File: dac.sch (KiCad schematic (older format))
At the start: 46 parts, among them U15 OPA4172, U4 OPA4172, U8 DAC8568C

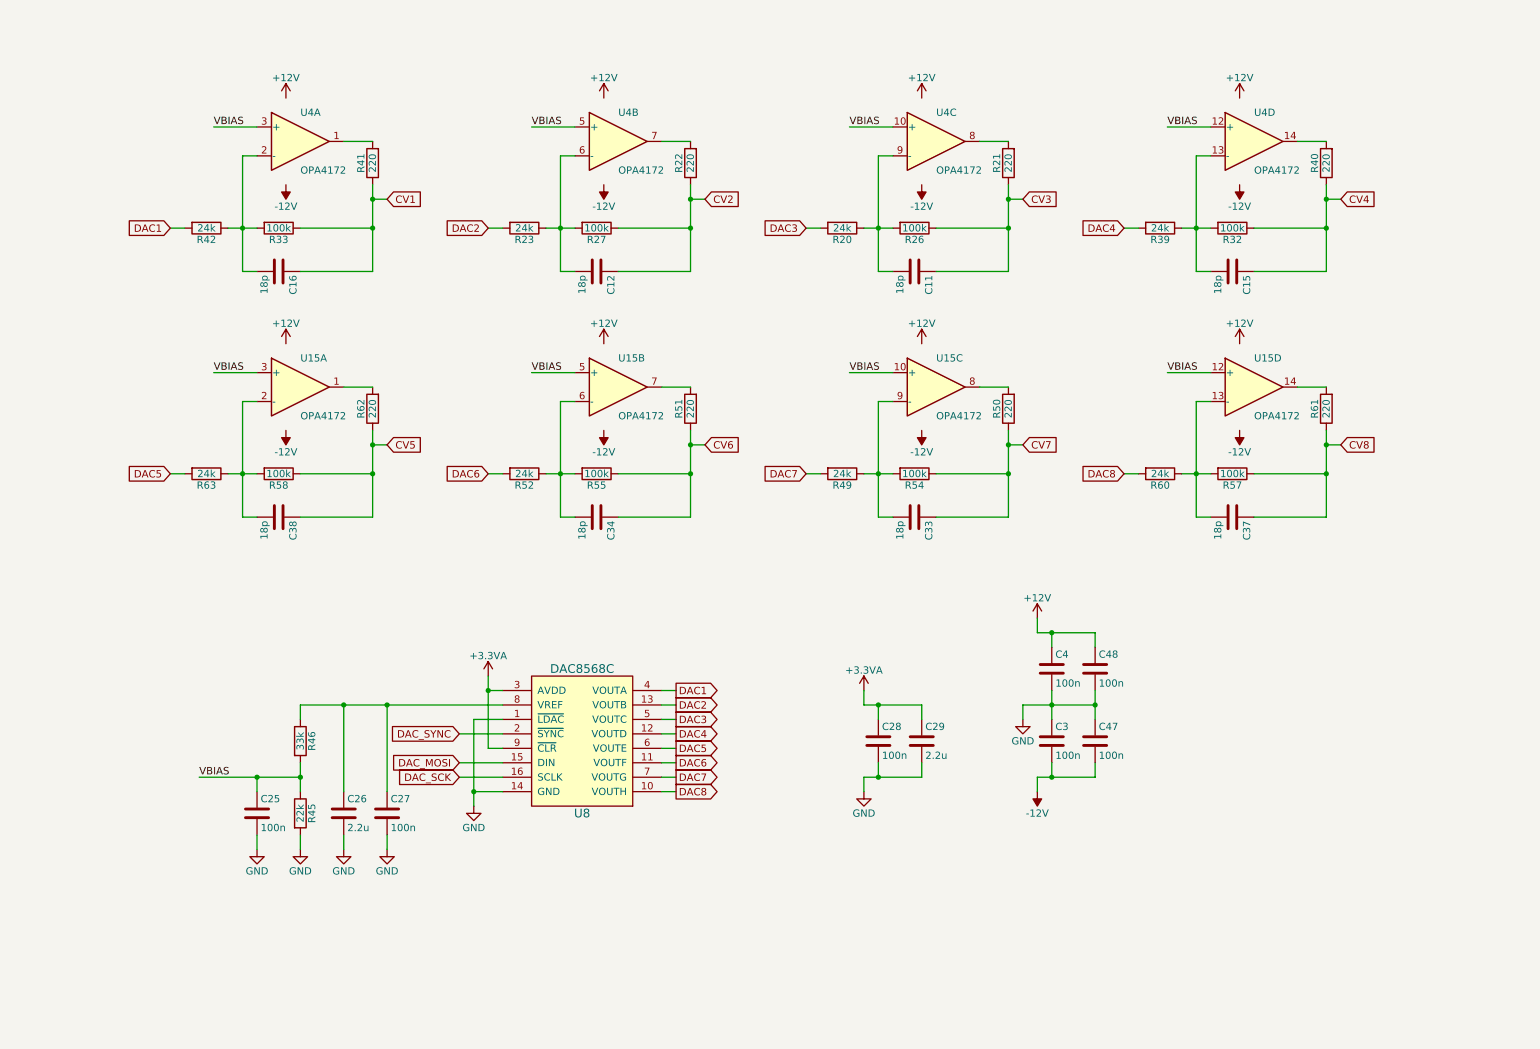
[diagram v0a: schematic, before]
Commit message: cleaned up schematics
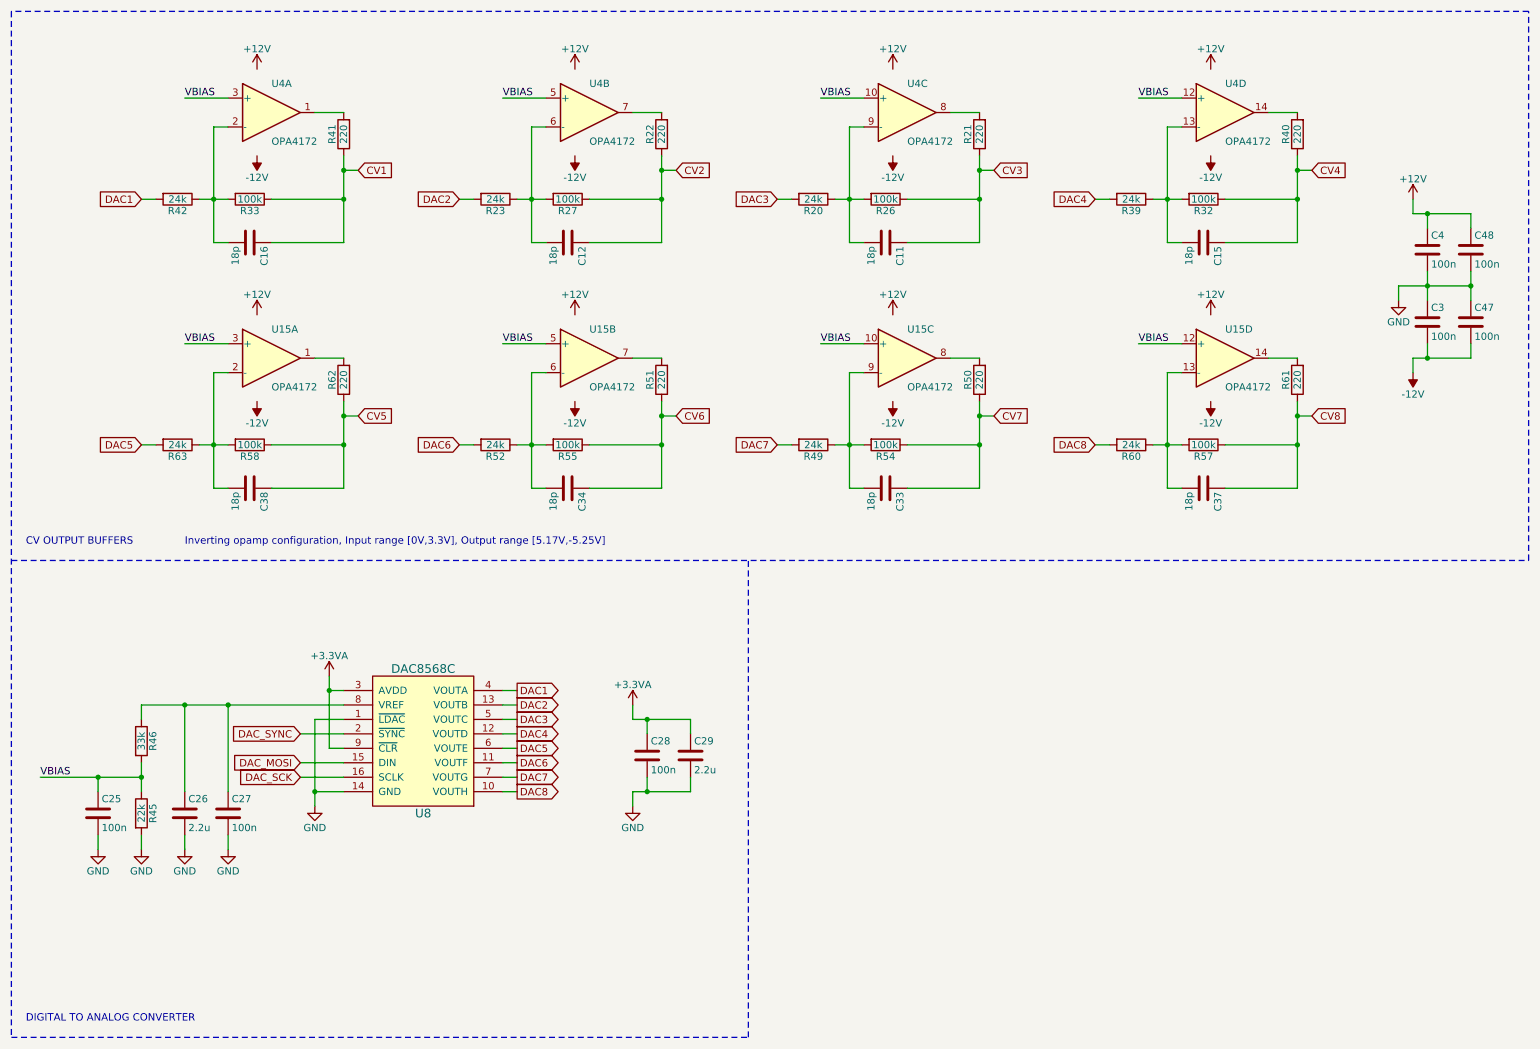
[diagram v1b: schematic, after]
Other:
- note added: "CV OUTPUT BUFFERS"
- note added: "DIGITAL TO ANALOG CONVERTER"
- note added: "Inverting opamp configuration, Input range [0V,3.3V], Output range [5.17V,-5.25V]"
- moved on the sheet: C11, C12, C15, C16, C25, C26, C27, C28, C29, C3, C33, C34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
